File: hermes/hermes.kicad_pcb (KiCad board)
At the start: 2 copper layers, 46 x 76 mm, 8 parts, among them U1 AHT20, U2 XIAO-RP2040-DIP

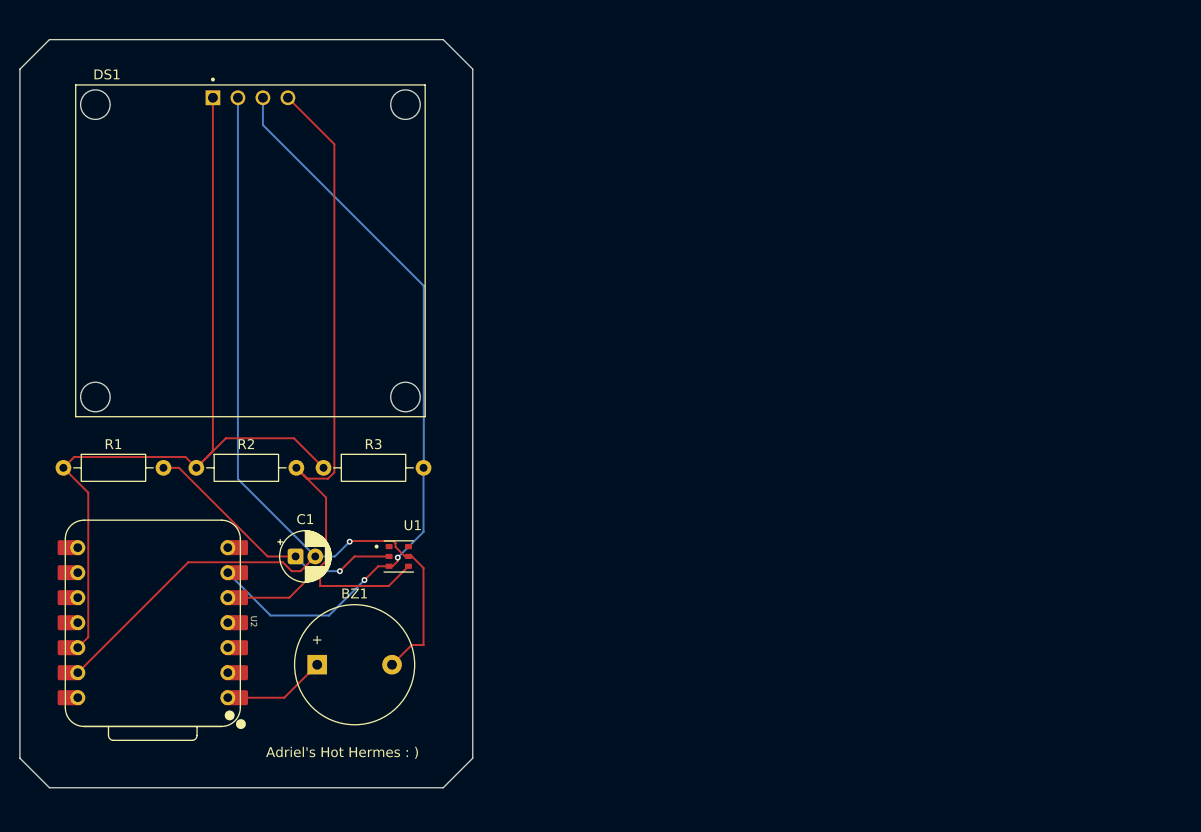
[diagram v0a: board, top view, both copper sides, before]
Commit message: done
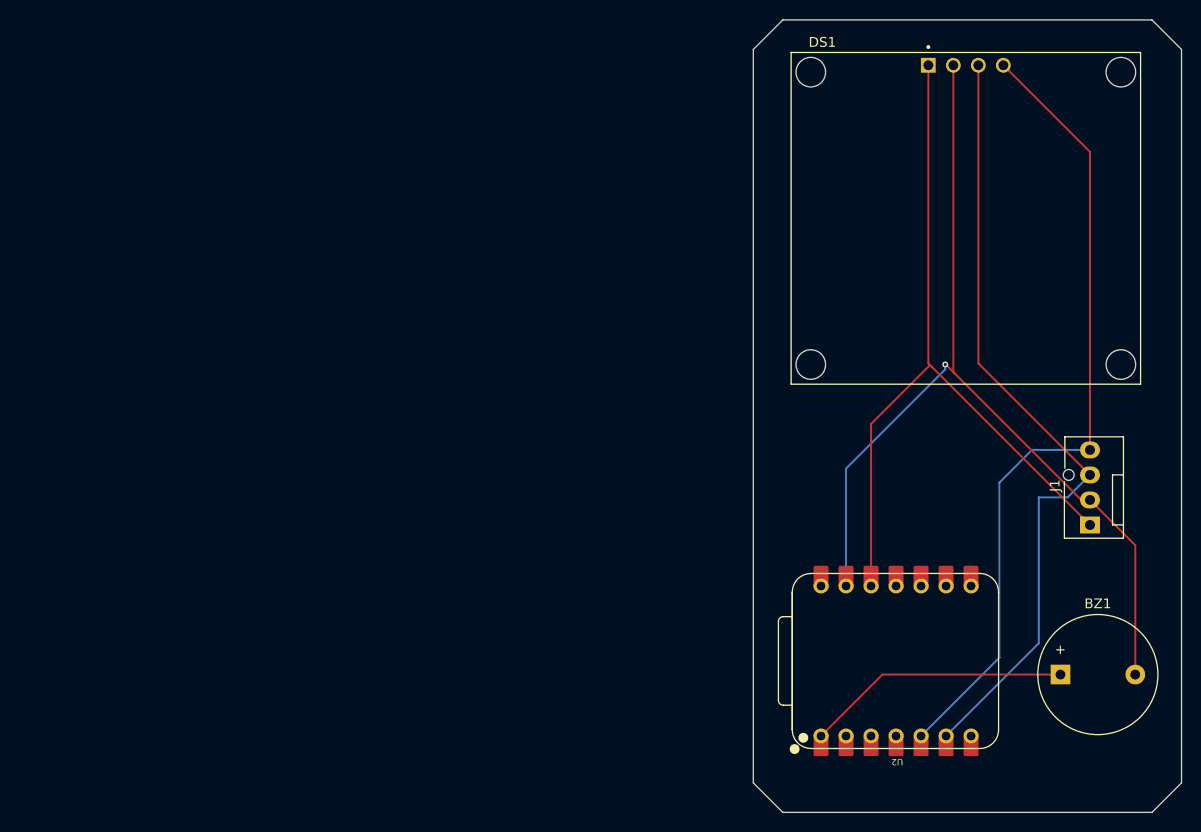
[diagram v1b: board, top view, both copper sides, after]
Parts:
- removed C1: 10u, Capacitor_THT:CP_Radial_D5.0mm_P2.00mm
- removed R1: 330, Resistor_THT:R_Axial_DIN0207_L6.3mm_D2.5mm_P10.16mm_Horizontal
- removed R2, R3: 4.7k, Resistor_THT:R_Axial_DIN0207_L6.3mm_D2.5mm_P10.16mm_Horizontal
- removed U1: AHT20, hermes-footprint:PSON100P300X300X110-6N
- added J1: Conn_01x04_Pin, Connector:FanPinHeader_1x04_P2.54mm_Vertical, F.Cu at (173.7, 98.8)
- moved U2 75.6 mm to (154.0, 112.6), turned to 180 degrees
- moved BZ1 75.5 mm to (170.7, 114.0)
- moved DS1 72.7 mm to (161.1, 67.7)
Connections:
- net Net-(DS1-SCK) renamed SCL
- net Net-(DS1-SDA) renamed SDA
- net Net-(DS1-VDD) renamed VDD
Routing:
- net Net-(U1-VDD): track 27.9 -> 0.00 mm, vias 1 -> 0
- net buzzer: track 10.5 -> 26.9 mm
- net VDD: track 87.9 -> 78.4 mm
- net GND: track 104.5 -> 98.2 mm
- net SDA: track 77.5 -> 82.3 mm
- net SCL: track 76.3 -> 80.6 mm, vias 2 -> 0
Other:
- board size 46 x 76 mm -> 43.5 x 80.5 mm
- board text removed: "Adriel's Hot Hermes : )"
